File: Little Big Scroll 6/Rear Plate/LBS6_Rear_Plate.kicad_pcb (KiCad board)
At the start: 2 copper layers, 57.2 x 85 mm, 6 parts

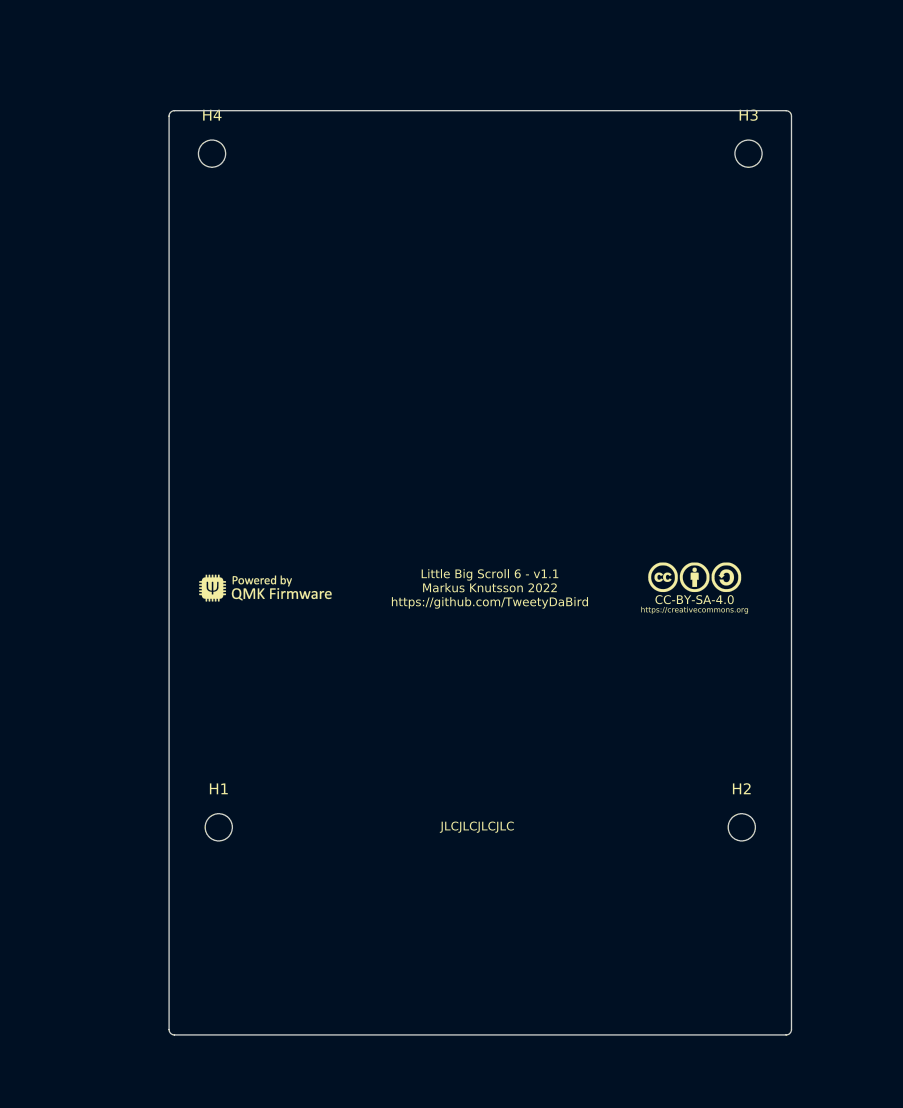
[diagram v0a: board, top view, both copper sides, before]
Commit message: LSB6 1.01
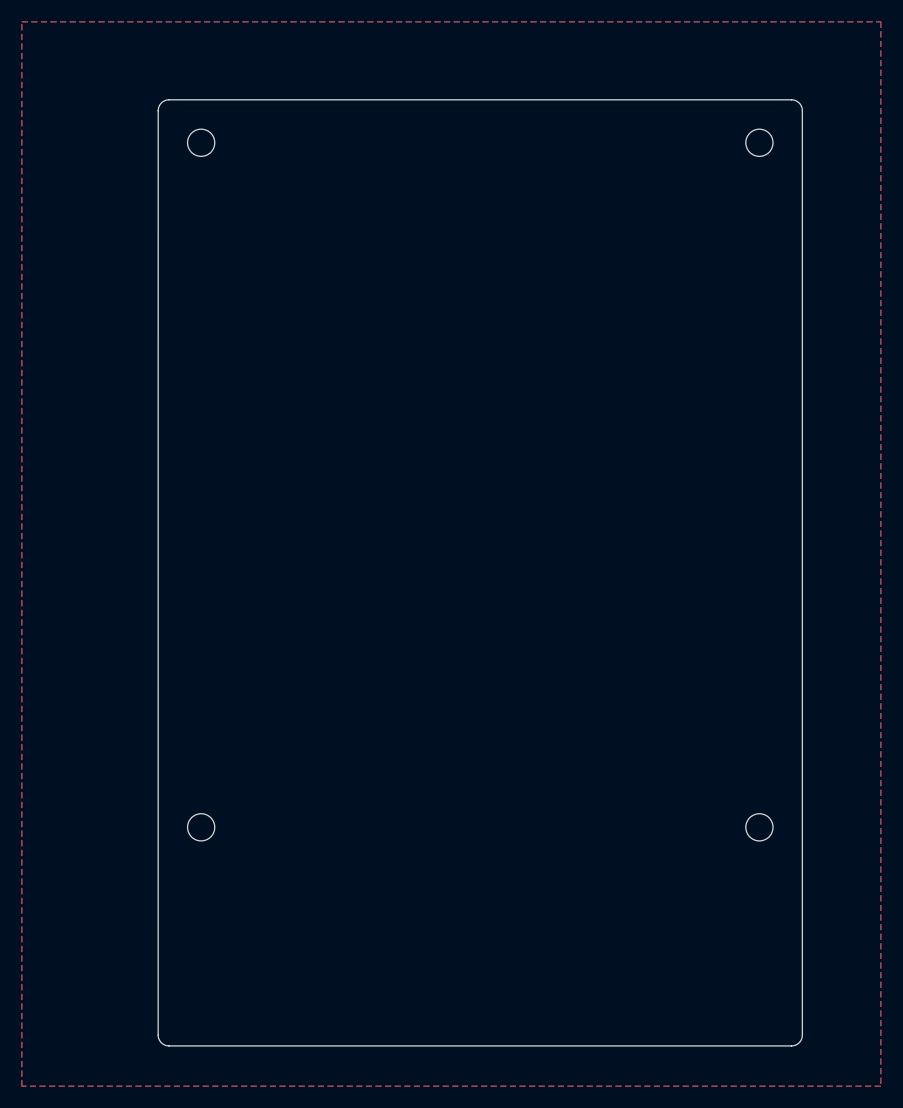
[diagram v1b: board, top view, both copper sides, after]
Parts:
- removed Lic1: CC-BY-SA-4.0, CC_Licensing:CC_BY_SA_40
- removed Logo1: QMK_Logo, QMK Logo:Powered_by_QMK
- H1, H2, H3, H4: value Hole_PCB_M2-Spacer -> Spacer_Plate
- moved H1 1.62 mm to (84.6, 112.7)
- moved H2 1.62 mm to (135.9, 112.7)
- moved H3 1.41 mm to (135.9, 49.7)
- moved H4 1.41 mm to (84.6, 49.7)
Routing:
- added copper zone on B.Cu, net (none)
- added copper zone on F.Cu, net (none)
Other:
- board size 57.2 x 85 mm -> 59.2 x 87 mm
- board text removed: "JLCJLCJLCJLC"
- board text removed: "Little Big Scroll 6 - v1.1 Markus Knutsson 2022 https://github.com/TweetyDaBird"
